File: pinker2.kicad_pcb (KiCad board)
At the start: 2 copper layers, 30 parts, among them J1 XLR3, Q1 BC549C, U1 OPA2134

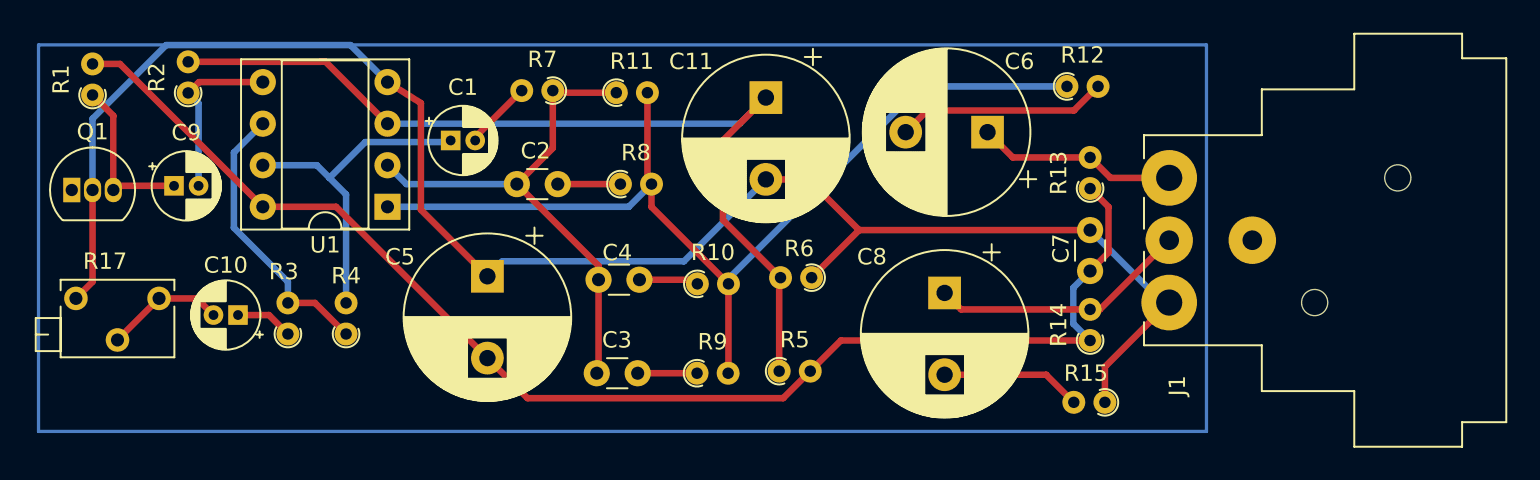
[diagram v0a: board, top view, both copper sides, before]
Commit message: almost complete
nudged some items, added a ground pour, linked the footprints to a local library (hopefully symbols live there too) added a pdf of the layout to help with visual diffs
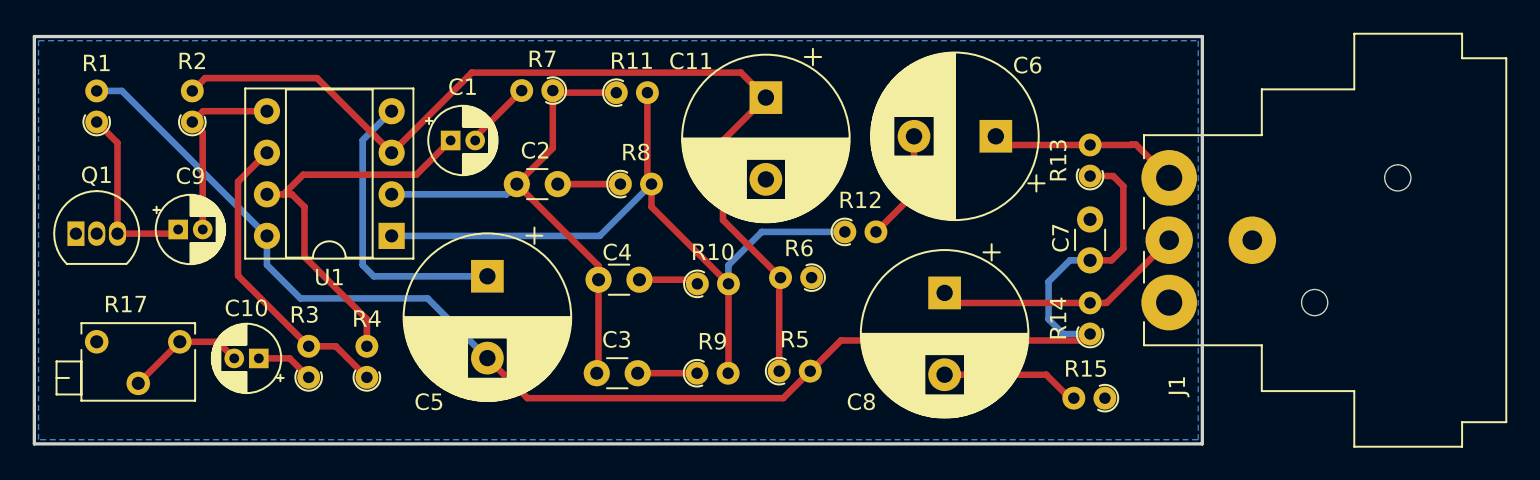
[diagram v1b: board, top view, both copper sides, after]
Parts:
- C1, C10, C9: footprint Capacitor_THT:CP_Radial_D4.0mm_P1.50mm -> Library:CP_Radial_D4.0mm_P1.50mm
- C11, C5, C6, C8: footprint Capacitor_THT:CP_Radial_D10.0mm_P5.00mm -> Library:CP_Radial_D10.0mm_P5.00mm
- C2, C3, C4, C7: footprint Capacitor_THT:C_Disc_D3.0mm_W1.6mm_P2.50mm -> Library:C_Disc_D3.0mm_W1.6mm_P2.50mm
- J1: footprint Connector_Audio:Jack_XLR_Neutrik_NC3MBH_Horizontal -> Library:Jack_XLR_Neutrik_NC3MBH_Horizontal
- Q1: footprint Package_TO_SOT_THT:TO-92_Inline -> Library:TO-92_Inline
- R1, R10, R11, R12, R13, R14, R15, R2, R3, R4, R5, R6, R7, R8, R9: footprint Resistor_THT:R_Axial_DIN0204_L3.6mm_D1.6mm_P1.90mm_Vertical -> Library:R_Axial_DIN0204_L3.6mm_D1.6mm_P1.90mm_Vertical
- R17: footprint Potentiometer_THT:Potentiometer_Bourns_3266X_Horizontal -> Library:Potentiometer_Bourns_3266X_Horizontal
- U1: footprint Package_DIP:DIP-8_W7.62mm_Socket -> Library:DIP-8_W7.62mm_Socket
- moved R12 16.2 mm to (174.0, 96.0)
- moved R17 2.94 mm to (133.3, 102.7)
- moved R4 2.94 mm to (144.8, 104.9)
- moved C10 2.94 mm to (138.2, 103.7)
- moved R3 2.94 mm to (141.2, 104.9)
- moved C9 2.68 mm to (133.2, 95.9)
- moved Q1 2.68 mm to (127.0, 96.1)
- moved U1 1.80 mm to (146.3, 96.3)
- moved R2 1.80 mm to (134.1, 89.3)
- moved R1 1.67 mm to (128.3, 89.3)
- moved R13 0.76 mm to (189.0, 92.6)
- moved C7 0.65 mm to (189.0, 95.2)
- moved C6 0.57 mm to (183.2, 90.2)
- moved R14 0.40 mm to (189.0, 102.3)
- moved R15 0.25 mm to (189.9, 106.2)
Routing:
- net Earth: track 106.0 -> 18.3 mm
- net Net-(R10-Pad2): track 61.8 -> 45.5 mm
- net Net-(C6-Pad2): track 12.9 -> 6.81 mm
- net Net-(C5-Pad2): track 82.3 -> 87.7 mm
- net Net-(C1-Pad1): track 20.8 -> 24.3 mm
- net Net-(C11-Pad1): track 56.8 -> 59.2 mm
- net Net-(R3-Pad2): track 17.4 -> 18.7 mm
- net Net-(C9-Pad1): track 10.1 -> 11.2 mm
- net Net-(C9-Pad2): track 10.8 -> 11.7 mm
- net Net-(C6-Pad1): track 12.3 -> 11.7 mm
- added copper zone on B.Cu, net Earth
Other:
- board outline added: 71.4 x 24.9 mm
